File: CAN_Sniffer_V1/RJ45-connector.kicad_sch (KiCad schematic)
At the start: 5 parts, among them J2 MTJ-88ARX1-FSM-LG, Q4 MMBT3906

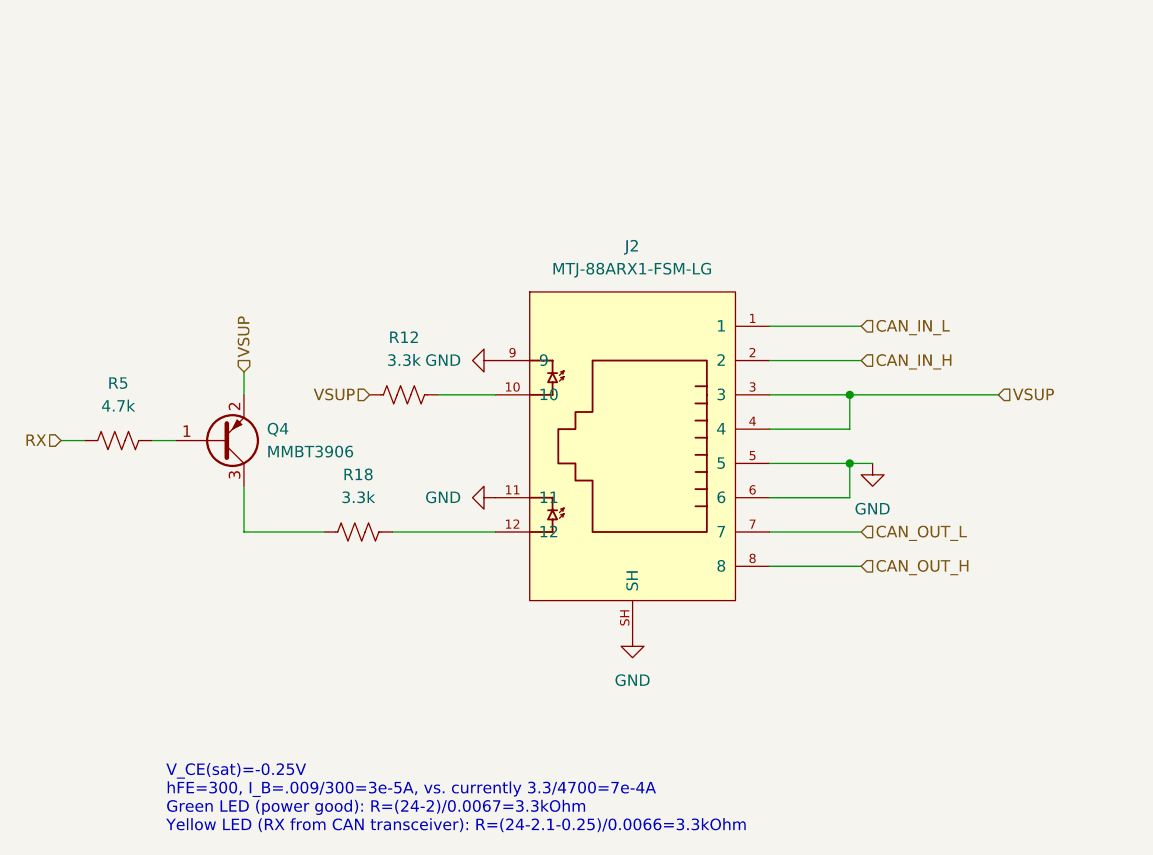
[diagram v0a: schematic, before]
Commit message: iteration 2 routing
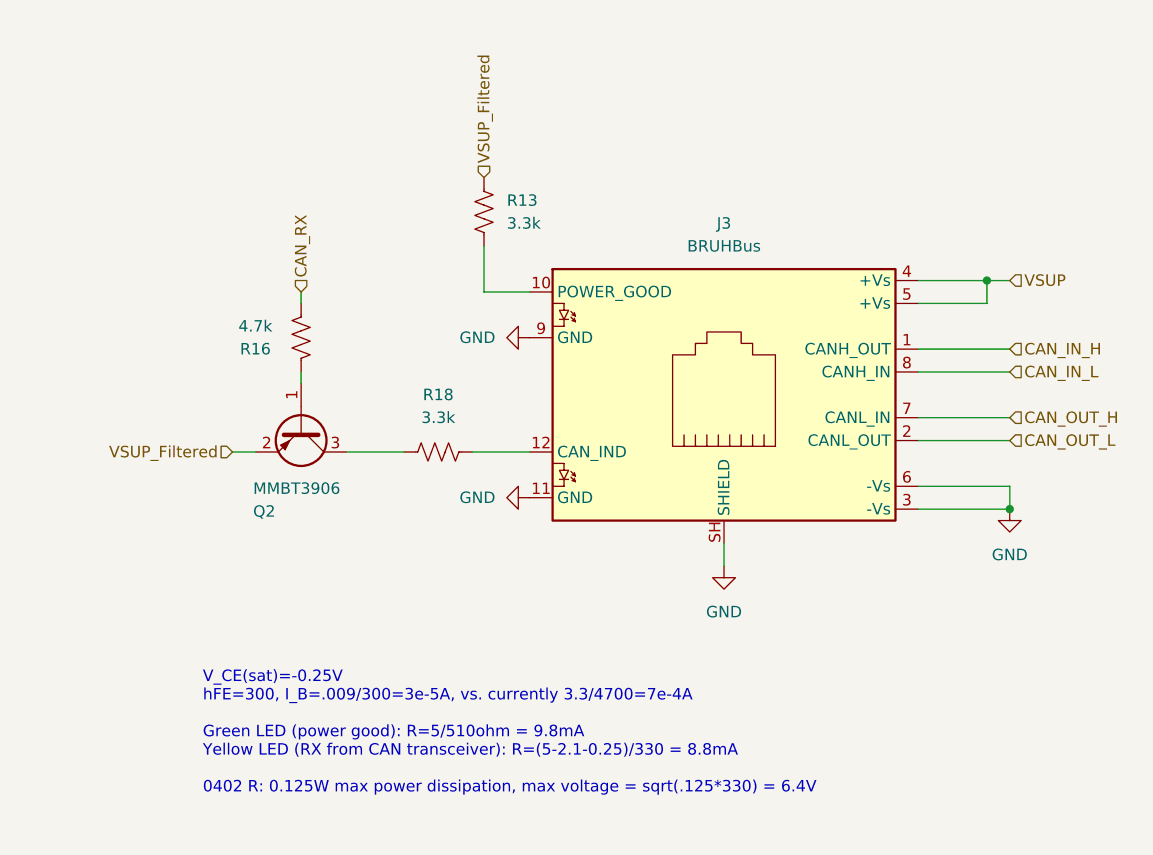
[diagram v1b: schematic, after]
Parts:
- removed J2: MTJ-88ARX1-FSM-LG, Connector_RJ:RJ45_Amphenol_RJHSE538X, symbol RJ45_Connector:MTJ-88ARX1-FSM-LG
- removed Q4: MMBT3906, Package_TO_SOT_SMD:SOT-23, symbol Transistor_BJT:MMBT3906
- removed R12, R18: 3.3k, Resistor_SMD:R_0402_1005Metric_Pad0.72x0.64mm_HandSolder, symbol bfr_resistors:RMCF0402FT3K30
- removed R5: 4.7k, Resistor_SMD:R_0603_1608Metric_Pad0.98x0.95mm_HandSolder, symbol bfr_resistors:RMCF0603FT4K70
- added J3: BRUHBus, Connector_RJ:RJ45_Amphenol_RJHSE538X, symbol bfr_connectors:BRUHbus
- added Q2: MMBT3906, Package_TO_SOT_SMD:SOT-23, symbol Transistor_BJT:MMBT3906
- added R13, R18: 3.3k, Resistor_SMD:R_0603_1608Metric_Pad0.98x0.95mm_HandSolder, symbol bfr_resistors:RMCF0603FT3K30
- added R16: 4.7k, Resistor_SMD:R_0603_1608Metric_Pad0.98x0.95mm_HandSolder, symbol bfr_resistors:RMCF0603FT4K70
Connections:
- net CAN_IN_H: now also J3.1 (CANH_OUT)
- net CAN_IN_L: now also J3.8 (CANH_IN)
- net CAN_OUT_H: now also J3.7 (CANL_IN)
- net CAN_OUT_L: now also J3.2 (CANL_OUT)
- net GND: now also J3.11 (GND), J3.3 (-Vs), J3.6 (-Vs), J3.9 (GND), J3.SH (SHIELD)
- net VSUP: now also J3.4 (+Vs), J3.5 (+Vs)
- new net: J3.10 (POWER_GOOD), R13.1
- new net: J3.12 (CAN_IND), R18.1
- new net: Q2.1 (B), R16.2
- new net: Q2.3 (C), R18.2
- new net CAN_RX: R16.1
- new net VSUP_Filtered: Q2.2 (E), R13.2
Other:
- note added: "V_CE(sat)=-0.25V hFE=300, I_B=.009/300=3e-5A, vs. currently 3.3/4700=7e-4A Green LED (power good): R=5/510ohm = 9.8mA Yellow LED (RX from CAN transceiver): R=(5-2.1-0.25)/330 = 8.8mA 0402 R: 0.125W max power dissipation, max voltage = sqrt(.125*330) = 6.4V"
- note removed: "V_CE(sat)=-0.25V hFE=300, I_B=.009/300=3e-5A, vs. currently 3.3/4700=7e-4A Green LED (power good): R=(24-2)/0.0067=3.3kOhm Yellow LED (RX from CAN transceiver): R=(24-2.1-0.25)/0.0066=3.3kOhm"
